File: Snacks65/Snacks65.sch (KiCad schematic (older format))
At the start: 149 parts, among them J1 Conn_02x03_Odd_Even, J2 Conn_01x04_Female, SW1 SW_PUSH, SW10 1U, SW11 1.25U, SW12 1U, SW13 1U, SW14 1U, SW15 1U, SW16 1.25U, SW17 1U, SW18 1U, SW19 1U, SW2 1U, SW20 1U, SW21 1U, SW22 1U, SW23 1U, SW24 1U, SW25 1U, SW26 1U, SW27 1U, SW28 1U, SW29 1U, SW3 1.5U, SW30 1U, SW31 1U, SW32 1U, SW33 6.25U, SW34 1U, SW35 1U, SW36 1U, SW37 1U, SW38 1U, SW39 1U, SW4 1.75U, SW40 1U, SW41 1U, SW42 1U, SW43 1U, SW44 1U, SW45 1U, SW46 1U, SW47 1U, SW48 1U, SW49 1U, SW5 1.25U, SW51 1U, SW52 1U, SW53 1U, SW54 1U, SW55 1.25U, SW56 1U, SW57 1U, SW58 2.25, SW59 1.75U, SW6 1.25U, SW60 1.25U, SW61 1U, SW62 1.5U, SW63 1U, SW64 1.25U, SW65 1U, SW66 2.25, SW67 2.75U, SW68 2U, SW69 1U, SW7 1U, SW70 1U, SW71 1U, SW72 1U, SW73 1U, SW74 1U, SW75 1U, SW76 1U, SW8 1U, SW9 1U, U1 ATmega32U4-AU, U2 USB2422-I_MJ, U3 AIC1221-33GY3TR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

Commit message: 7/24
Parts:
- removed C1, C10, C8: 1uF, Capacitor_SMD:C_0805_2012Metric, symbol Device:C_Small
- removed C11, C12, C2, C3, C5, C9: 100nF, Capacitor_SMD:C_0805_2012Metric, symbol Device:C_Small
- removed C13, C6: 4.7uF, Capacitor_SMD:C_0805_2012Metric, symbol Device:C_Small
- removed C14: 10uF, Capacitor_SMD:C_0805_2012Metric, symbol Device:C_Small
- removed C4, C7: 18pF, Capacitor_SMD:C_0805_2012Metric, symbol Device:C_Small
- removed D29: LED, LED_THT:LED_D3.0mm, symbol Device:LED
- removed D39, D40: BAV70, Package_TO_SOT_SMD:SOT-23, symbol Diode:BAV70
- removed F1: ASMD1206-200, Fuse:Fuse_1206_3216Metric, symbol Device:Fuse
- removed J1: Conn_02x03_Odd_Even, Connector_PinHeader_2.54mm:PinHeader_2x03_P2.54mm_Vertical, symbol Connector_Generic:Conn_02x03_Odd_Even
- removed J2: Conn_01x04_Female, random-keyboard-parts:JST-SR-4, symbol Connector:Conn_01x04_Female
- removed R10: 12kΩ, Resistor_SMD:R_0805_2012Metric, symbol Device:R_Small
- removed R11: 2.2k, Resistor_SMD:R_0805_2012Metric, symbol Device:R_Small
- removed R3, R4: 10kΩ, Resistor_SMD:R_0805_2012Metric, symbol Device:R_Small
- removed R5: 330Ω, Resistor_SMD:R_0805_2012Metric, symbol Device:R_Small
- removed R6, R7: 5.1kΩ, Resistor_SMD:R_0805_2012Metric, symbol Device:R_Small
- removed R8: 100kΩ, Resistor_SMD:R_0805_2012Metric, symbol Device:R_Small
- removed R9: 100k, Resistor_SMD:R_0805_2012Metric, symbol Device:R_Small
- removed SW1: SW_PUSH, random-keyboard-parts:SKQG-1155865, symbol kbd:SW_PUSH
- removed SW73, SW76: 1U, MX_Alps_Hybrid:MX-1U-NoLED, symbol Base65-rescue:SW_Push-Switch
- removed U1: ATmega32U4-AU, Package_QFP:TQFP-44_10x10mm_P0.8mm, symbol MCU_Microchip_ATmega:ATmega32U4-AU
- removed U2: USB2422-I_MJ, symbol usb2422:USB2422-I_MJ
- removed U3: AIC1221-33GY3TR, symbol Regulator_Linear:AZ1117-3.3
- removed USB1: HRO-TYPE-C-31-M-12, Type-C:HRO-TYPE-C-31-M-12-HandSoldering, symbol keebio:HRO-TYPE-C-31-M-12
- removed Y1: Resonator_Small, proj_local:Resonator_SMD_muRata_CSTxExxV-3Pin_3.0x1.1mm_HandSoldering_Compact, symbol Device:Resonator_Small
- removed Y2: Crystal_GND24, keyboard_parts:FA-238, symbol Device:Crystal_GND24
- added A1: Adafruit_Feather_32u4_BluefruitLE, feather:Adafruit_Feather, symbol MCU_Module:Adafruit_Feather_32u4_BluefruitLE
- added J1: Sensor Connector, Connector_FFC-FPC:Hirose_FH12-6S-0.5SH_1x06-1MP_P0.50mm_Horizontal, symbol Connector:Conn_01x06_Female
- added SW1: SW_SPDT, Custom_Footprints:Slide_Switch_SPDT_ThroughHole, symbol Switch:SW_SPDT
- R1, R2: value 22Ω -> 4.7k
- SW10, SW11, SW12, SW13, SW14, SW15, SW16, SW17, SW18, SW19, SW2, SW20, SW21, SW22, SW23, SW24, SW25, SW26, SW27, SW28, SW29, SW3, SW30, SW31, SW32, SW33, SW34, SW35, SW36, SW37, SW38, SW39, SW4, SW40, SW41, SW42, SW43, SW44, SW45, SW46, SW47, SW48, SW49, SW5, SW51, SW52, SW53, SW54, SW55, SW56, SW57, SW58, SW59, SW6, SW60, SW61, SW62, SW63, SW64, SW65, SW66, SW67, SW68, SW69, SW7, SW70, SW71, SW72, SW74, SW75, SW8, SW9: symbol Base65-rescue:SW_Push-Switch -> Snacks65-rescue:SW_Push-Switch-Base65-rescue
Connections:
- net labels added: +3V3, EN, RDY, SCL, SDA
- net labels removed: +5V, COL8, DOWN1_5V, DOWN1_D+, DOWN1_D-, DOWN2_D+, DOWN2_D-, ENABLE_1, ENABLE_2, FLAG_1, FLAG_2, MCU_D+, MCU_D-, MCU_VBUS, MISO, MOSI, PD+, PD-, SCK, TRACKPAD_D+, TRACKPAD_D-, TRACKPAD_VBUS, USBXTAL1, USBXTAL2, USB_UP_D+, USB_UP_D-, VBUS_UP, VBUS_UP3.3V, VBUS_UP5V, VDD33
- wire segments 399 -> 263
- no-connect marks 4 -> 5
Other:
- note removed: "USB C"
- moved on the sheet: D32, D36, D37

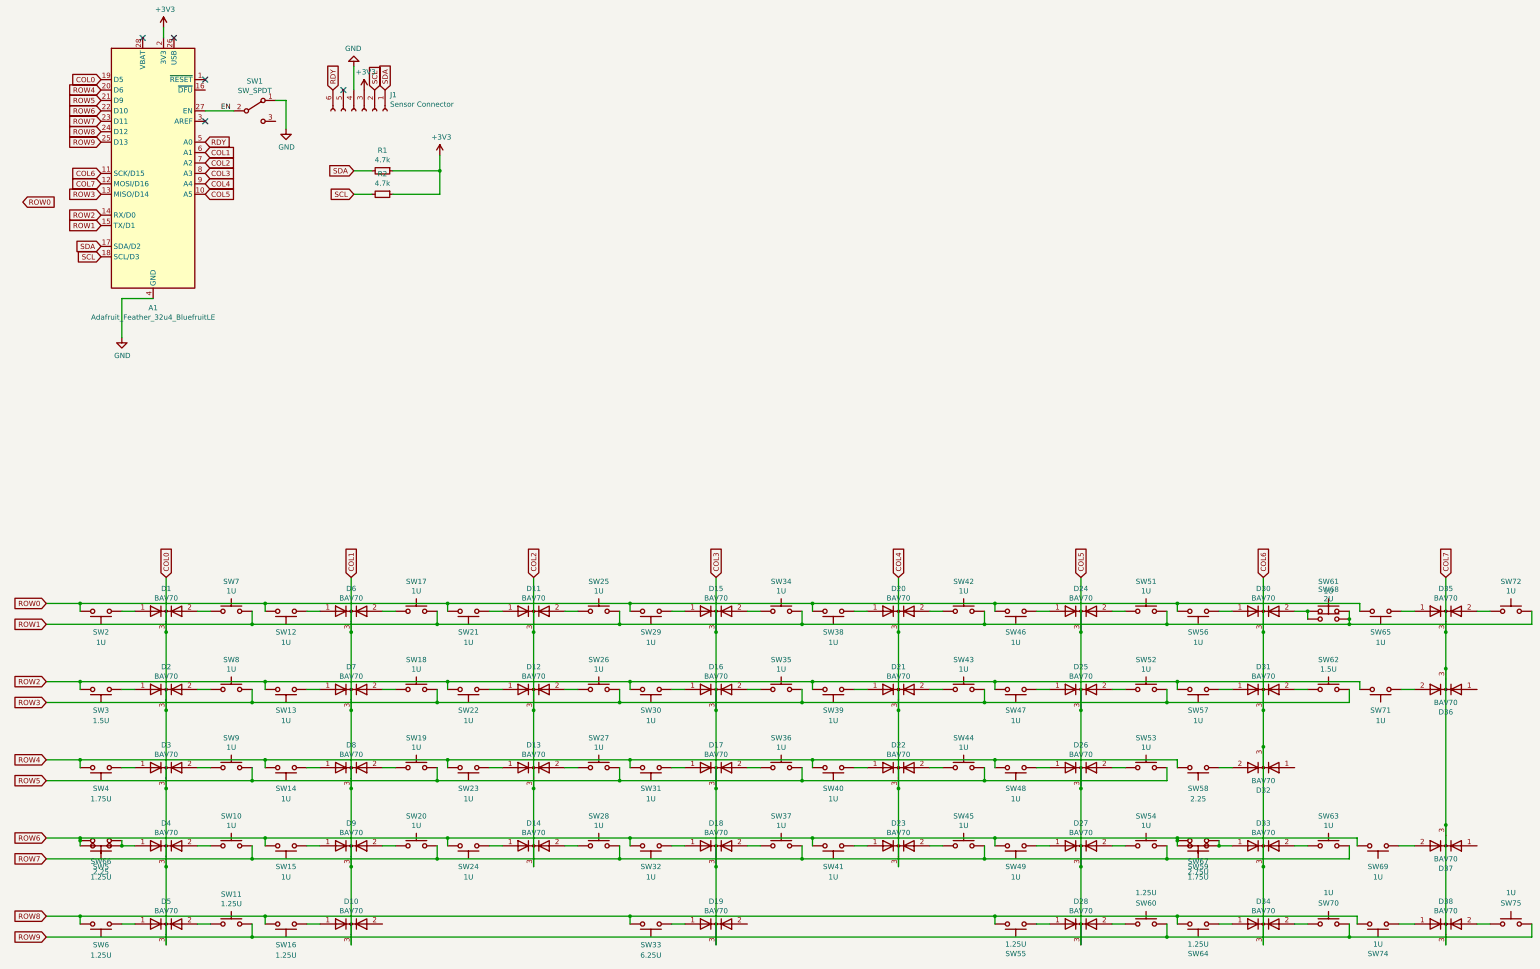
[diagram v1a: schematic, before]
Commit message: 7-27
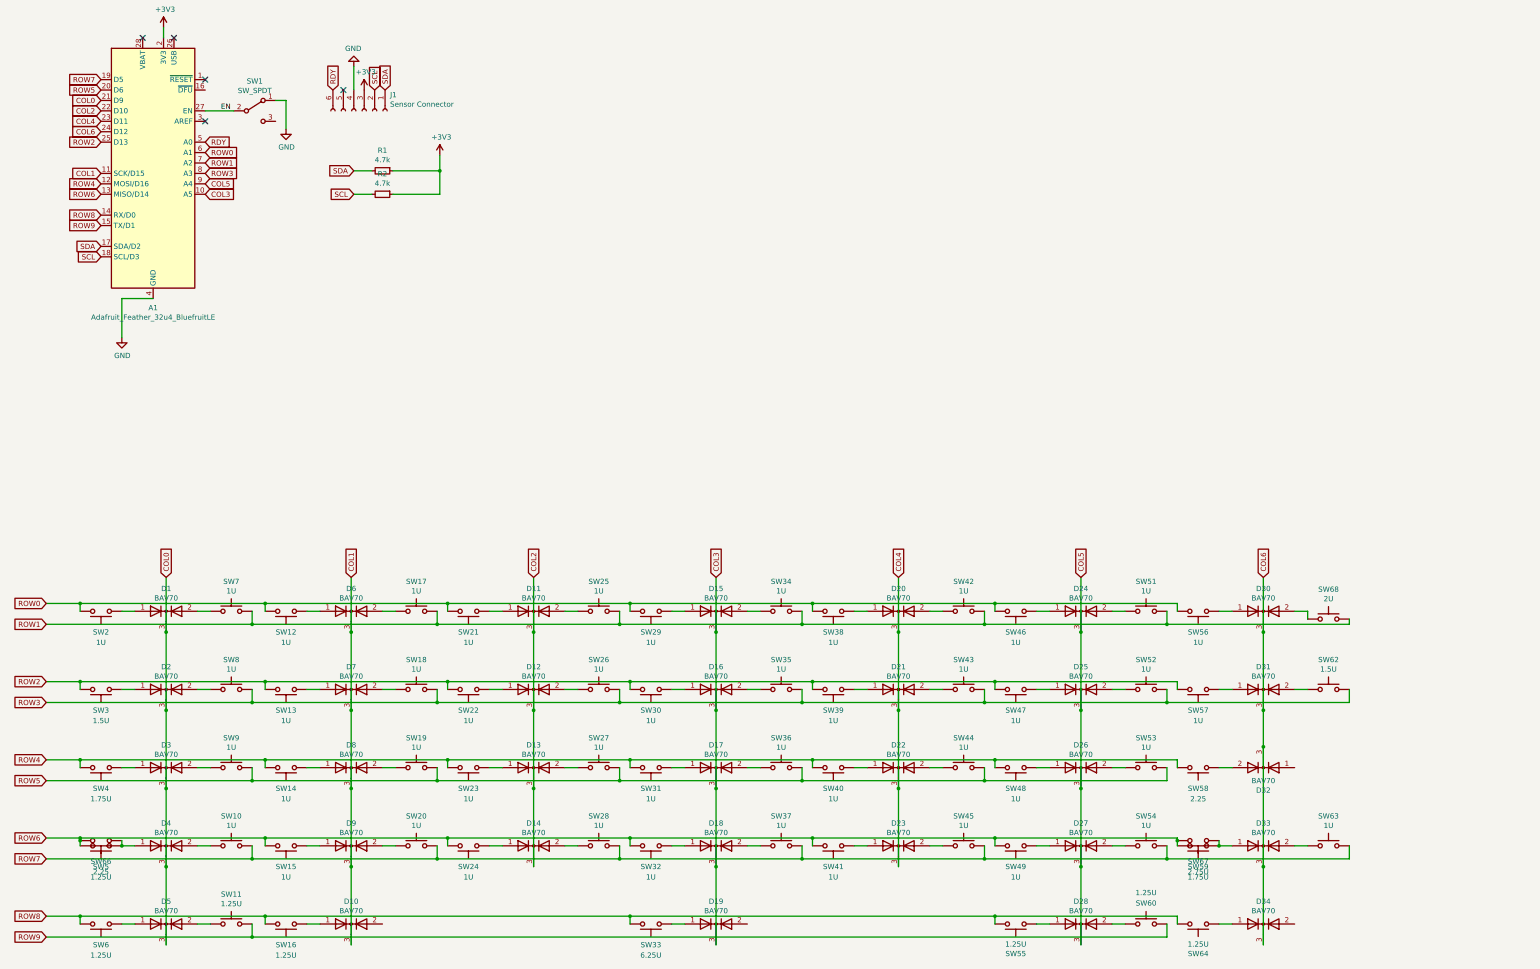
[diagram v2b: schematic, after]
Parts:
- removed D35, D36, D37, D38: BAV70, Package_TO_SOT_SMD:SOT-23, symbol Diode:BAV70
- removed SW61, SW65, SW69, SW70, SW71, SW72, SW74, SW75: 1U, MX_Alps_Hybrid:MX-1U-NoLED, symbol Snacks65-rescue:SW_Push-Switch-Base65-rescue
- D1, D10, D11, D12, D13, D14, D15, D16, D17, D18, D19, D2, D20, D21, D22, D23, D24, D25, D26, D27, D28, D3, D30, D31, D32, D33, D34, D4, D5, D6, D7, D8, D9: LCSC Part# (none) -> C68978; Mfr (none) -> Changjiang Electronics Tech (CJ); Part# (none) -> BAV70
- J1: LCSC Part# (none) -> C202118; Mfr (none) -> HRS(Hirose); Part# (none) -> FH12-6S-0.5SH(55)
- R1, R2: LCSC Part# (none) -> C17673; Mfr (none) -> UNI-ROYAL(Uniroyal Elec); Part# (none) -> 0805W8F4701T5E
- SW1: Field4 C698225 -> (none); LCSC Part# (none) -> C698225; Mfr (none) -> USAKRO; Part# (none) -> SS-12D03-G4
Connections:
- net COL7 is gone; now on net ROW4: A1.12 (MOSI/D16)
- net COL0: now also A1.21 (D9); no longer A1.19 (D5)
- net COL1: now also A1.11 (SCK/D15); no longer A1.6 (A1)
- net COL2: now also A1.22 (D10); no longer A1.7 (A2)
- net COL3: now also A1.10 (A5); no longer A1.8 (A3)
- net COL4: now also A1.23 (D11); no longer A1.9 (A4)
- net COL5: now also A1.9 (A4); no longer A1.10 (A5)
- net COL6: now also A1.24 (D12); no longer A1.11 (SCK/D15)
- net ROW0: now also A1.6 (A1)
- net ROW1: now also A1.7 (A2); no longer A1.15 (TX/D1)
- net ROW2: now also A1.25 (D13); no longer A1.14 (RX/D0)
- net ROW3: now also A1.8 (A3); no longer A1.13 (MISO/D14)
- net ROW4: no longer A1.20 (D6)
- net ROW5: now also A1.20 (D6); no longer A1.21 (D9)
- net ROW6: now also A1.13 (MISO/D14); no longer A1.22 (D10)
- net ROW7: now also A1.19 (D5); no longer A1.23 (D11)
- net ROW8: now also A1.14 (RX/D0); no longer A1.24 (D12)
- net ROW9: now also A1.15 (TX/D1); no longer A1.25 (D13)

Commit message: 7/27
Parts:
- A1: symbol MCU_Module:Adafruit_Feather_32u4_BluefruitLE -> Snacks65-rescue:Adafruit_Feather_32u4_BluefruitLE-MCU_Module
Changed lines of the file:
@@
 RDY
 $Comp
-L MCU_Module:Adafruit_Feather_32u4_BluefruitLE A1
+L Snacks65-rescue:Adafruit_Feather_32u4_BluefruitLE-MCU_Module A1
 U 1 1 60FDCBB8
 P 2025 2025

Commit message: 8/29
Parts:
- added D29, D35, D36, D37: BAV70, Package_TO_SOT_SMD:SOT-23, symbol Diode:BAV70
- added SW50, SW61, SW65, SW69, SW70, SW71: 1U, MX_Alps_Hybrid:MX-1U-NoLED, symbol Snacks65-rescue:SW_Push-Switch-Base65-rescue
- added U1: MCP23017_SP, Package_DIP:DIP-28_W7.62mm, symbol Interface_Expansion:MCP23017_SP
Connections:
- net +3V3: now also U1.9 (VDD)
- net COL1: now also U1.1 (GPB0); no longer A1.11 (SCK/D15)
- net COL2: now also A1.14 (RX/D0); no longer A1.22 (D10)
- net COL4: now also A1.9 (A4); no longer A1.23 (D11)
- net COL5: now also A1.23 (D11); no longer A1.9 (A4)
- net COL6: now also A1.8 (A3); no longer A1.24 (D12)
- net GND: now also U1.10 (VSS)
- net ROW0: now also SW61.2
- net ROW2: now also SW65.2
- net ROW3: now also A1.24 (D12); no longer A1.8 (A3)
- net ROW4: now also U1.3 (GPB2); no longer A1.12 (MOSI/D16)
- net ROW6: now also SW69.2, U1.4 (GPB3); no longer A1.13 (MISO/D14)
- net ROW8: now also A1.22 (D10), SW70.2; no longer A1.14 (RX/D0)
- net ROW9: now also SW50.2, SW71.2, U1.5 (GPB4); no longer A1.15 (TX/D1)
- net SCL: now also U1.12 (SCK)
- net SDA: now also U1.13 (SDA)
- net at D34.2 (A): now also SW50.1
- new net: D29.2 (A), SW61.1
- new net: D35.2 (A), SW65.1
- new net: D36.2 (A), SW69.1
- new net: D37.1 (A), SW70.1
- new net: D37.2 (A), SW71.1
- new net COL7: D29.3 (K), D35.3 (K), D36.3 (K), D37.3 (K), U1.2 (GPB1)
- new net INTB: A1.15 (TX/D1), U1.19 (INTB)
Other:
- moved on the sheet: J1, R1, R2
